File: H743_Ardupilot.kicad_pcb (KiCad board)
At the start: 2 copper layers, 36.5 x 36.5 mm, 142 parts, among them J1 Conn_01x04, J10 Conn_01x03, J11 Conn_01x03, J12 10067099-200LF, J2 Conn_01x04, J3 Conn_01x04, J4 Conn_01x06, J5 Conn_01x04, J6 Conn_01x04, J7 Conn_01x04, J8 Conn_01x04, J9 Conn_01x04, Q1 AO3400A, U10 LSM6DSV16X, U12 BMP581, U2 STM32H743VIT6, U8 ZX-SH1.0-4PWT, U9 BMI088

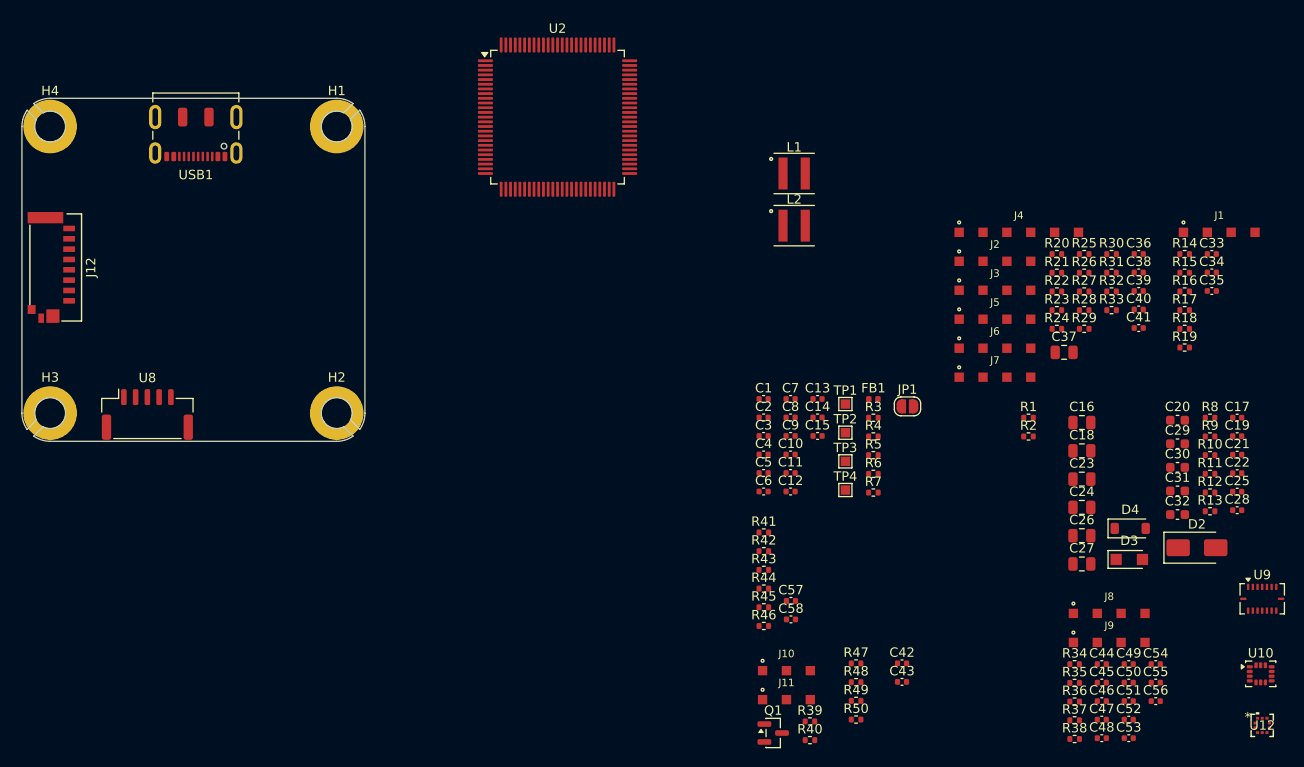
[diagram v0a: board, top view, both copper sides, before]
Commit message: ok
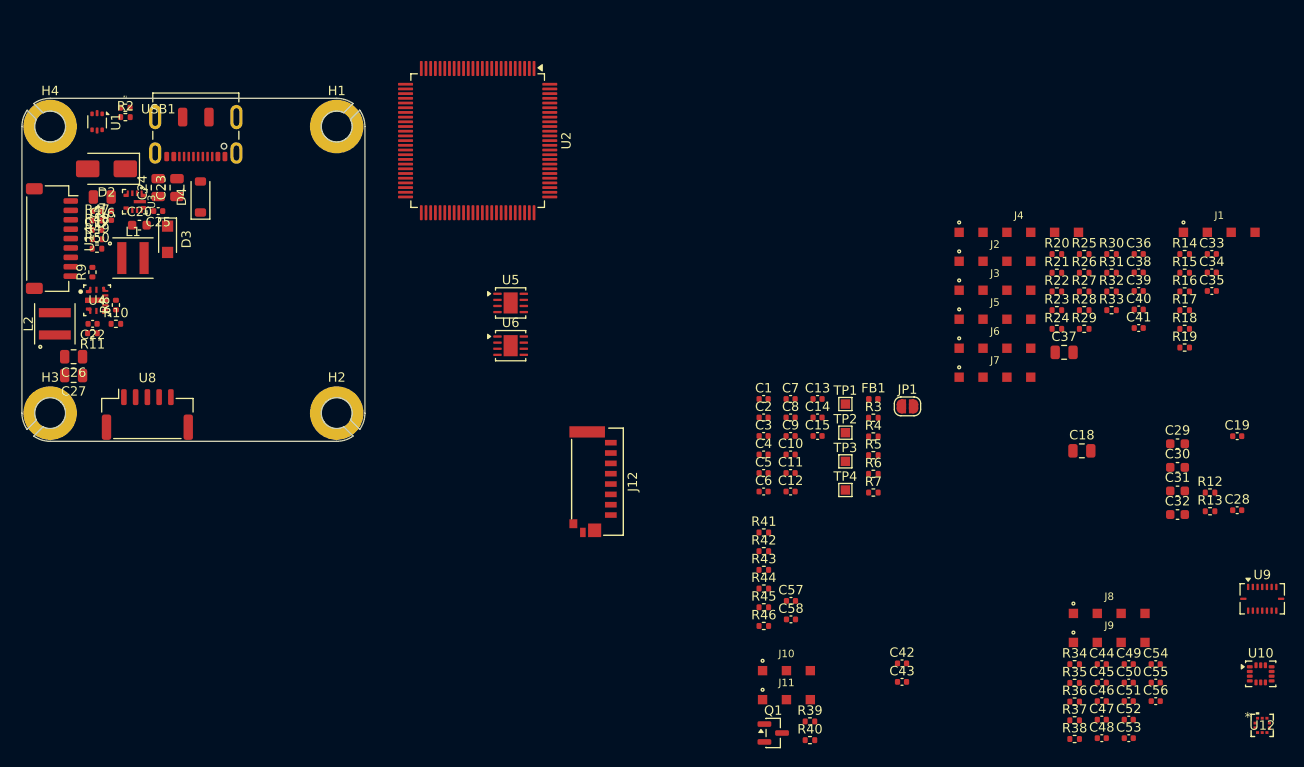
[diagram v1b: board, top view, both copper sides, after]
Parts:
- added U1: Power_Protection:USBLC6-2P6, Package_TO_SOT_SMD:SOT-666, F.Cu at (82.5, 88.0)
- added U14: ZX-SH1.0-8PWT, Connector_JST:JST_SH_SM09B-SRSS-TB_1x09-1MP_P1.00mm_Horizontal, F.Cu at (77.7, 100.4)
- added U3: LMR43620R5RPER, H743_Custom:TI_RPE0009B_VQFN-HR-9_2x2mm, F.Cu at (86.5, 96.5)
- added U4: LMR604303SRAKRQ1, H743_Custom:TI_RAK0009A_WQFN-HR-9_2.5x2.0mm, F.Cu at (82.5, 107.0)
- added U5: AP7361C-33FGE-7, Package_DFN_QFN:DFN-8-1EP_3x3mm_P0.65mm_EP1.5x2.25mm, F.Cu at (126.5, 107.3)
- added U6: AP7361C-33FGE-7, Package_DFN_QFN:DFN-8-1EP_3x3mm_P0.65mm_EP1.5x2.25mm, F.Cu at (126.5, 111.8)
- USB1: footprint Connector_USB:USB_C_Receptacle_JAE_DX07S016JA1R1500 -> H743_Custom:JAE_DX07S016JA1R1500_16P
- moved C17 123.3 mm to (82.5, 97.5), turned to 180 degrees
- moved D2 122.9 mm to (83.5, 93.0), turned to 180 degrees
- moved C22 122.8 mm to (82.0, 109.5), turned to 180 degrees
- moved C21 122.5 mm to (84.0, 98.0), turned to 90 degrees
- moved R9 120.2 mm to (82.0, 104.0), turned to 90 degrees
- moved R11 119.9 mm to (82.0, 110.5), turned to 180 degrees
- moved C25 118.7 mm to (89.0, 97.5), turned to 180 degrees
- moved R10 117.3 mm to (84.5, 109.5)
- moved R8 117.1 mm to (84.5, 107.5), turned to 90 degrees
- moved C20 112.4 mm to (87.0, 99.0)
- moved C27 109.2 mm to (80.0, 115.0), turned to 180 degrees
- moved C26 109.0 mm to (80.0, 113.0), turned to 180 degrees
- moved D3 107.9 mm to (90.0, 100.5), turned to -90 degrees
- moved C16 107.0 mm to (83.0, 96.0), turned to 180 degrees
- moved D4 105.0 mm to (93.5, 96.0), turned to 90 degrees
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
